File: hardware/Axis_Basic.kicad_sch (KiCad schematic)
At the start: 15 parts, among them U2 2MB Flash, U3 AP2112-3.3, X2 32.768

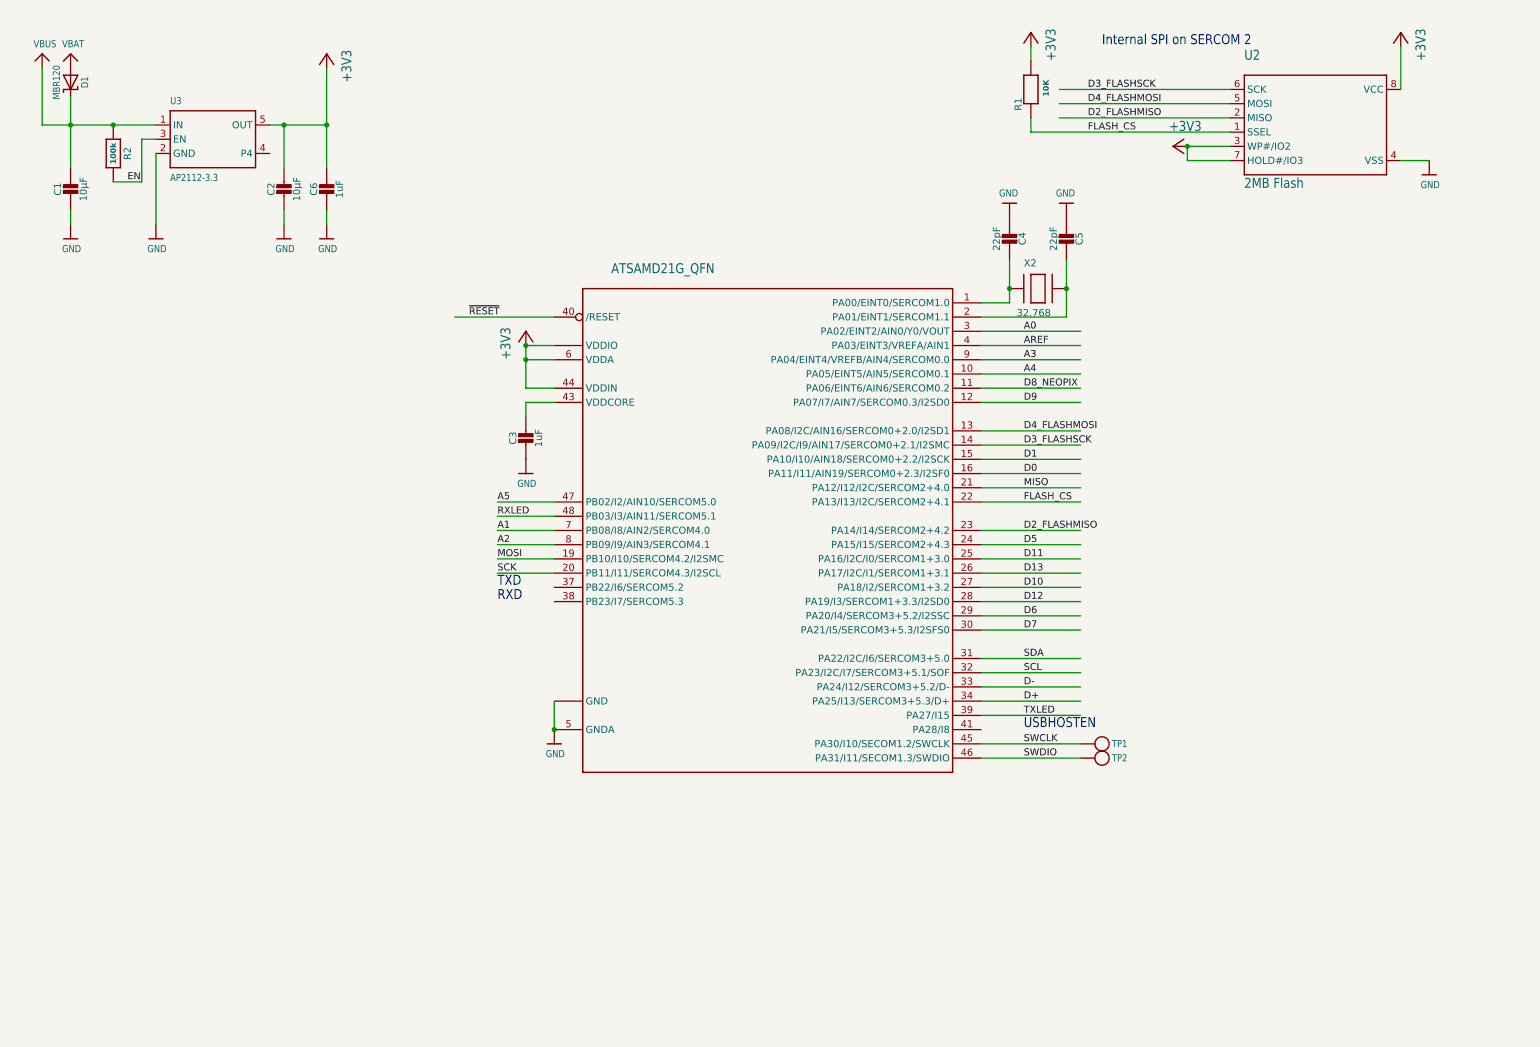
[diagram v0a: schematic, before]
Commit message: compontents placed
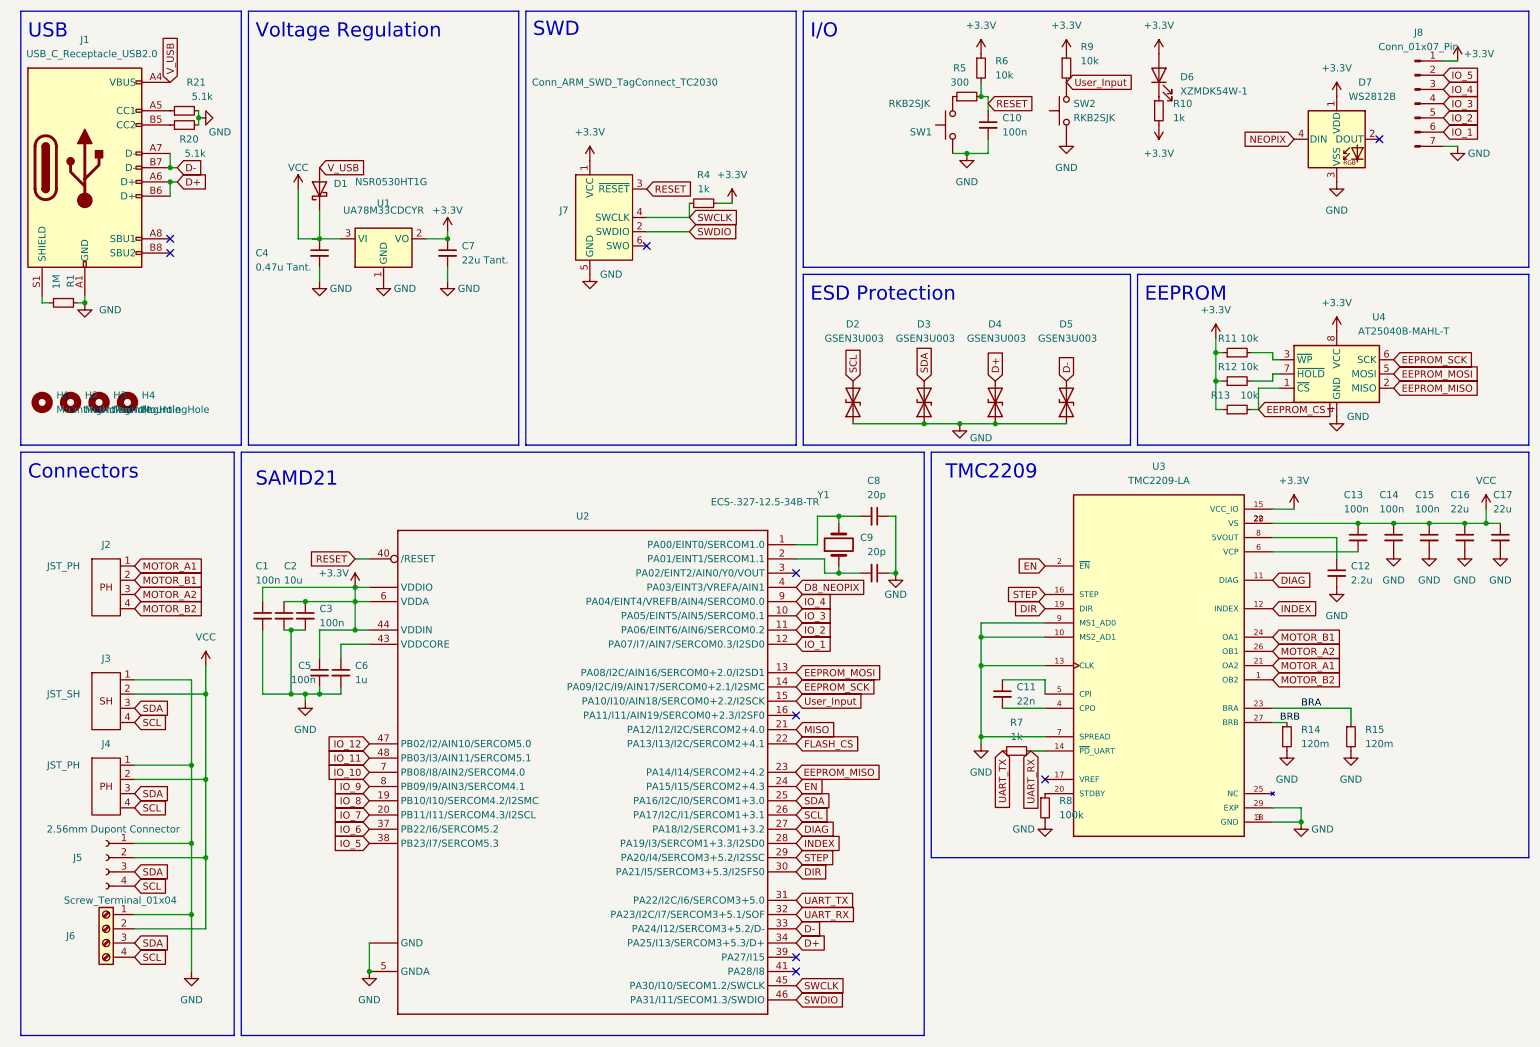
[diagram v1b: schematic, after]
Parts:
- removed C1, C2: 10µF, Adafruit Feather M0 Express:0805-NO, symbol Adafruit Feather M0 Express-eagle-import:CAP_CERAMIC0805-NOOUTLINE
- removed C3, C6: 1uF, Adafruit Feather M0 Express:0603-NO, symbol Adafruit Feather M0 Express-eagle-import:CAP_CERAMIC0603_NO
- removed C4, C5: 22pF, Adafruit Feather M0 Express:0603-NO, symbol Adafruit Feather M0 Express-eagle-import:CAP_CERAMIC0603_NO
- removed D1: MBR120, Adafruit Feather M0 Express:SOD-123, symbol Adafruit Feather M0 Express-eagle-import:DIODE-SCHOTTKYSOD-123
- removed R1: 10K, Adafruit Feather M0 Express:0603-NO, symbol Adafruit Feather M0 Express-eagle-import:RESISTOR_0603_NOOUT
- removed R2: 100k, Adafruit Feather M0 Express:0603-NO, symbol Adafruit Feather M0 Express-eagle-import:RESISTOR_0603_NOOUT
- removed TP1, TP2: TESTPOINTROUND1.5MM, Adafruit Feather M0 Express:TESTPOINT_ROUND_1.5MM, symbol Adafruit Feather M0 Express-eagle-import:TESTPOINTROUND1.5MM
- removed U$1: ATSAMD21G_QFN, Adafruit Feather M0 Express:TQFN48_7MM, symbol Adafruit Feather M0 Express-eagle-import:ATSAMD21G_QFN
- removed U2: 2MB Flash, Adafruit Feather M0 Express:SOIC8_208MIL, symbol Adafruit Feather M0 Express-eagle-import:SPIFLASH_SOIC8208MIL
- removed U3: AP2112-3.3, Adafruit Feather M0 Express:SOT23-5, symbol Adafruit Feather M0 Express-eagle-import:VREG_SOT23-5
- removed X2: 32.768, Adafruit Feather M0 Express:XTAL3215, symbol Adafruit Feather M0 Express-eagle-import:XTAL-3.2X1.5
- added C1, C10, C13, C14, C15, C3, C5: 100n, Capacitor_SMD:C_0402_1005Metric, symbol Device:C_Small
- added C11: 22n, Capacitor_SMD:C_0402_1005Metric, symbol Device:C_Small
- added C12: 2.2u, Capacitor_SMD:C_0402_1005Metric, symbol Device:C_Small
- added C16, C17: 22u, Capacitor_SMD:C_0805_2012Metric, symbol Device:C_Small
- added C2: 10u, Capacitor_SMD:C_0402_1005Metric, symbol Device:C_Small
- added C4: 0.47u Tant., Capacitor_SMD:C_0402_1005Metric, symbol Device:C_Small
- added C6: 1u, Capacitor_SMD:C_0402_1005Metric, symbol Device:C_Small
- added C7: 22u Tant., Capacitor_SMD:C_0402_1005Metric, symbol Device:C_Small
- added C8, C9: 20p, Capacitor_SMD:C_0402_1005Metric, symbol Device:C_Small
- added D1: NSR0530HT1G, Diode_SMD:D_SOD-323, symbol Diode:NSR0340HT1G
- added D2, D3, D4, D5: GSEN3U003, Diode_SMD:D_0603_1608Metric, symbol Device:D_TVS
- added D6: XZMDK54W-1, LED_SMD:LED_0603_1608Metric, symbol Device:LED
- added D7: WS2812B, LED_SMD:LED_WS2812B_PLCC4_5.0x5.0mm_P3.2mm, symbol LED:WS2812B
- added H1, H2, H3, H4: MountingHole, MountingHole:MountingHole_3.2mm_M3, symbol Mechanical:MountingHole
- added J1: USB_C_Receptacle_USB2.0, GCT_USB4120-03-C_REVA:GCT_USB4120-03-C_REVA, symbol Connector:USB_C_Receptacle_USB2.0
- added J2, J4: JST_PH, Connector_JST:JST_PH_B4B-PH-K_1x04_P2.00mm_Vertical, symbol JST:JST_PH_4pin
- added J3: JST_SH, Connector_JST:JST_SH_BM04B-SRSS-TB_1x04-1MP_P1.00mm_Vertical, symbol JST:JST_SH_4pin
- added J5: 2.56mm Dupont Connector, Connector_PinSocket_2.54mm:PinSocket_1x04_P2.54mm_Vertical, symbol Connector:Conn_01x04_Socket
- added J6: Screw_Terminal_01x04, Screw_Terminal:EBBA-04-C-SS-BU, symbol Connector:Screw_Terminal_01x04
- added J7: Conn_ARM_SWD_TagConnect_TC2030, Connector_PinHeader_1.27mm:PinHeader_2x03_P1.27mm_Vertical_SMD, symbol Connector:Conn_ARM_SWD_TagConnect_TC2030
- added J8: Conn_01x07_Pin, Connector_PinSocket_2.54mm:PinSocket_1x07_P2.54mm_Vertical, symbol Connector:Conn_01x07_Pin
- added R1: 1M, Resistor_SMD:R_0402_1005Metric, symbol Device:R_Small
- added R10, R4, R7: 1k, Resistor_SMD:R_0402_1005Metric, symbol Device:R_Small
- added R11, R12, R13, R6, R9: 10k, Resistor_SMD:R_0402_1005Metric, symbol Device:R_Small
- added R14, R15: 120m, Resistor_SMD:R_1206_3216Metric, symbol Device:R_Small
- added R20, R21: 5.1k, Resistor_SMD:R_0402_1005Metric, symbol Device:R_Small
- added R5: 300, Resistor_SMD:R_0402_1005Metric, symbol Device:R_Small
- added R8: 100k, Resistor_SMD:R_0402_1005Metric, symbol Device:R_Small
- added SW1, SW2: RKB2SJK, Push_Button:button_RKB2SJK250SMTR LFS, symbol Switch:SW_Push
- added U1: UA78M33CDCYR, Package_TO_SOT_SMD:SOT-223-3_TabPin2, symbol Regulator_Linear:AP1117-33
- added U2: ~, Package_QFP:TQFP-48-1EP_7x7mm_P0.5mm_EP3.5x3.5mm, symbol SAMD21:ATSAMD21G18A-AUT
- added U3: TMC2209-LA, Package_DFN_QFN:QFN-28-1EP_5x5mm_P0.5mm_EP3.35x3.35mm_ThermalVias, symbol TMC2209-LA:TMC2209-LA
- added U4: AT25040B-MAHL-T, Package_DFN_QFN:DFN-8-1EP_3x2mm_P0.5mm_EP1.3x1.5mm, symbol Memory_EEPROM:AT25xxx-MA
- added Y1: ECS-.327-12.5-34B-TR, Crystal:Crystal_SMD_G8-2Pin_3.2x1.5mm, symbol Device:Crystal
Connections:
- net D+: now also D4.2 (A2), J1.A6 (D+), J1.B6 (D+), U2.34 (PA25/I13/SERCOM3+5.3/D+)
- net D-: now also D5.2 (A2), J1.A7 (D-), J1.B7 (D-), U2.33 (PA24/I12/SERCOM3+5.2/D-)
- net D8_NEOPIX: now also U2.4 (PA03/EINT3/VREFA/AIN1)
- net EN: now also U2.24 (PA15/I15/SERCOM2+4.3), U3.2 (~{EN})
- net FLASH_CS: now also U2.22 (PA13/I13/I2C/SERCOM2+4.1)
- net GND: now also C1.2, C10.2, C12.2, C14.2, C15.2, C16.2, C17.2, C2.2, C3.2, C4.2, C5.2, C6.2, C7.2, C8.1, C9.1, D2.1 (A1), D3.1 (A1), D4.1 (A1), D5.1 (A1), D7.3 (VSS), J1.A1 (GND), J1.A12 (GND), J1.B1 (GND), J1.B12 (GND), J3.1, J4.1, J5.1 (Pin_1), J6.1 (Pin_1), J7.5 (GND), J8.7 (Pin_7), R1.1, R14.2, R15.2, R20.2, R21.2, R8.2, SW1.1, SW2.1, U1.1 (GND), U2.18 (GND), U2.35 (GND), U2.42 (GND), U2.5 (GNDA), U2.THERMAL (GND), U3.10 (MS2_AD1), U3.13 (CLK), U3.18 (GND), U3.29 (EXP), U3.3 (GND), U3.7 (SPREAD), U3.9 (MS1_AD0), U4.4 (GND), U4.9 (GND)
- net MISO: now also U2.21 (PA12/I12/I2C/SERCOM2+4.0)
- net SCL: now also D2.2 (A2), J3.4, J4.4, J5.4 (Pin_4), J6.4 (Pin_4), U2.26 (PA17/I2C/I1/SERCOM1+3.1)
- net SDA: now also D3.2 (A2), J3.3, J4.3, J5.3 (Pin_3), J6.3 (Pin_3), U2.25 (PA16/I2C/I0/SERCOM1+3.0)
- net SWCLK: now also J7.4 (SWCLK), R4.1, U2.45 (PA30/I10/SECOM1.2/SWCLK)
- net SWDIO: now also J7.2 (SWDIO), U2.46 (PA31/I11/SECOM1.3/SWDIO)
- new net: D6.1 (K), R10.1
- new net: C8.2, U2.1 (PA00/EINT0/SERCOM1.0), Y1.2
- new net: C9.2, U2.2 (PA01/EINT1/SERCOM1.1), Y1.1
- new net: C6.1, U2.43 (VDDCORE)
- new net: C13.2, U3.6 (VCP)
- new net: J1.A5 (CC1), R21.1
- new net: R11.2, U4.3 (~{WP})
- new net: J1.B5 (CC2), R20.1
- new net: J1.S1 (SHIELD), R1.2
- new net: R8.1, U3.20 (STDBY)
- new net: C11.2, U3.4 (CPO)
- new net: C11.1, U3.5 (CPI)
- new net: C12.1, U3.8 (5VOUT)
- new net: R12.2, U4.7 (~{HOLD})
- new net: R5.1, SW1.2
- new net +3.3V: C1.1, C2.1, C3.1, C5.1, C7.1, D6.2 (A), D7.1 (VDD), J7.1 (VCC), J8.1 (Pin_1), R10.2, R11.1, R12.1, R13.1, R4.2, R6.1, R9.1, U1.2 (VO), U2.17 (VDDIO), U2.36 (VDDIO), U2.44 (VDDIN), U2.6 (VDDA), U3.15 (VCC_IO), U4.8 (VCC)
- new net BRA: R15.1, U3.23 (BRA)
- new net BRB: R14.1, U3.27 (BRB)
- new net DIAG: U2.27 (PA18/I2/SERCOM1+3.2), U3.11 (DIAG)
- new net DIR: U2.30 (PA21/I5/SERCOM3+5.3/I2SFS0), U3.19 (DIR)
- new net EEPROM_CS: R13.2, U4.1 (~{CS})
- new net EEPROM_MISO: U2.23 (PA14/I14/SERCOM2+4.2), U4.2 (MISO)
- new net EEPROM_MOSI: U2.13 (PA08/I2C/AIN16/SERCOM0+2.0/I2SD1), U4.5 (MOSI)
- new net EEPROM_SCK: U2.14 (PA09/I2C/I9/AIN17/SERCOM0+2.1/I2SMC), U4.6 (SCK)
- new net INDEX: U2.28 (PA19/I3/SERCOM1+3.3/I2SD0), U3.12 (INDEX)
- new net IO_1: J8.6 (Pin_6), U2.12 (PA07/I7/AIN7/SERCOM0.3/I2SD0)
- new net IO_10: U2.7 (PB08/I8/AIN2/SERCOM4.0)
- new net IO_11: U2.48 (PB03/I3/AIN11/SERCOM5.1)
- new net IO_12: U2.47 (PB02/I2/AIN10/SERCOM5.0)
- new net IO_2: J8.5 (Pin_5), U2.11 (PA06/EINT6/AIN6/SERCOM0.2)
- new net IO_3: J8.4 (Pin_4), U2.10 (PA05/EINT5/AIN5/SERCOM0.1)
- new net IO_4: J8.3 (Pin_3), U2.9 (PA04/EINT4/VREFB/AIN4/SERCOM0.0)
- new net IO_5: J8.2 (Pin_2), U2.38 (PB23/I7/SERCOM5.3)
- new net IO_6: U2.37 (PB22/I6/SERCOM5.2)
- new net IO_7: U2.20 (PB11/I11/SERCOM4.3/I2SCL)
- new net IO_8: U2.19 (PB10/I10/SERCOM4.2/I2SMC)
- new net IO_9: U2.8 (PB09/I9/AIN3/SERCOM4.1)
- new net MOTOR_A1: J2.1, U3.21 (OA2)
- new net MOTOR_A2: J2.3, U3.26 (OB1)
- new net MOTOR_B1: J2.2, U3.24 (OA1)
- new net MOTOR_B2: J2.4, U3.1 (OB2)
- new net NEOPIX: D7.4 (DIN)
- new net RESET: C10.1, J7.3 (~{RESET}), R5.2, R6.2, U2.40 (/RESET)
- new net STEP: U2.29 (PA20/I4/SERCOM3+5.2/I2SSC), U3.16 (STEP)
- new net UART_RX: R7.2, U2.32 (PA23/I2C/I7/SERCOM3+5.1/SOF), U3.14 (~{PD}_UART)
- new net UART_TX: R7.1, U2.31 (PA22/I2C/I6/SERCOM3+5.0)
- new net User_Input: R9.2, SW2.2, U2.15 (PA10/I10/AIN18/SERCOM0+2.2/I2SCK)
- new net VCC: C13.1, C14.1, C15.1, C16.1, C17.1, C4.1, D1.1 (K), J3.2, J4.2, J5.2 (Pin_2), J6.2 (Pin_2), U1.3 (VI), U3.22 (VS), U3.28 (VS)
- new net V_USB: D1.2 (A), J1.A4 (VBUS), J1.A9 (VBUS), J1.B4 (VBUS), J1.B9 (VBUS)
- no-connect marks 0 -> 9
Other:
- note added: "Connectors"
- note added: "EEPROM"
- note added: "ESD Protection"
- note added: "I/O"
- note added: "SAMD21"
- note added: "SWD"
- note added: "TMC2209"
- note added: "USB"
- note added: "Voltage Regulation"
- note removed: "Internal SPI on SERCOM 2"
- note removed: "RXD"
- note removed: "TXD"
- note removed: "USBHOSTEN"
